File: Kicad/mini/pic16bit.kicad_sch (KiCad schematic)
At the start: 12 parts, among them K101 PE-450-4X6X-BLACK

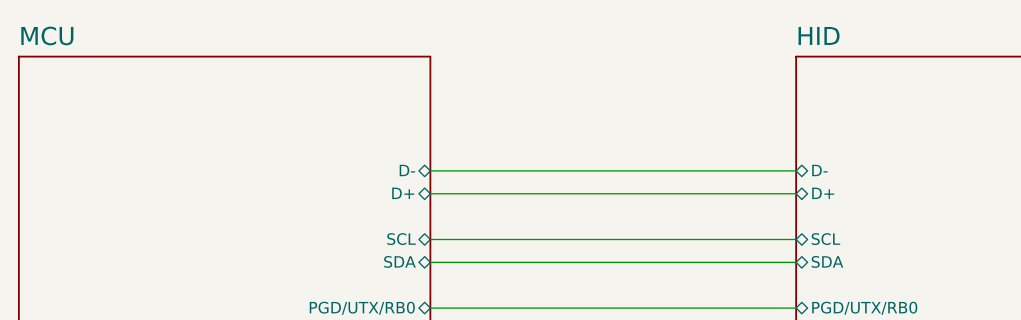
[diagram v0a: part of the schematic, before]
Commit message: Up
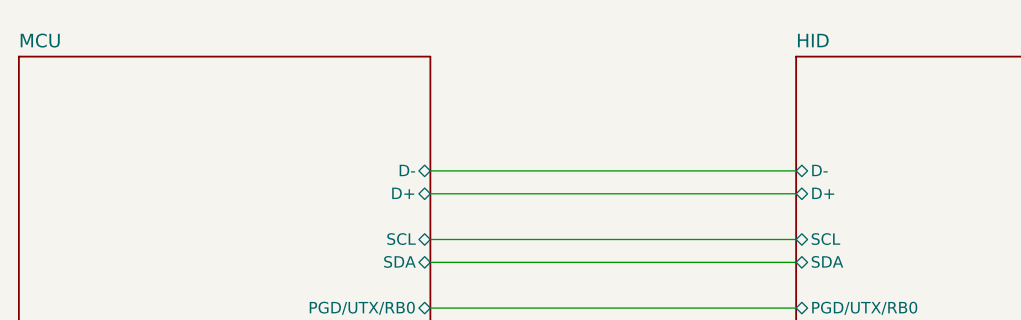
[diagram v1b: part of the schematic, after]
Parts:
- H101, H102, H103, H104, JP101, JP102, JP103, JP104, JP105, JP106, JP107, K101: now in the parts list
